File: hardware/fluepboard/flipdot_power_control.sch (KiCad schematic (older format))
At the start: 6 parts, among them IC3 SI4835DDY-T1-E3, Q2 BC847

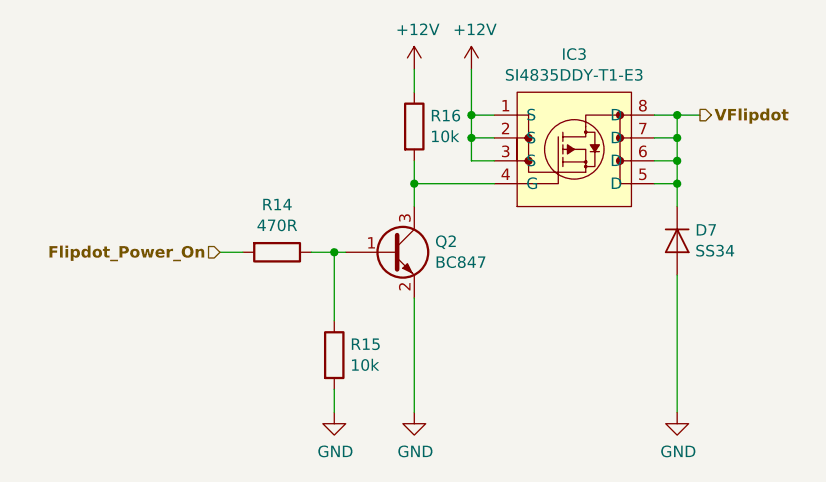
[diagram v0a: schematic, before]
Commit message: Commit jlcpcb compatible version
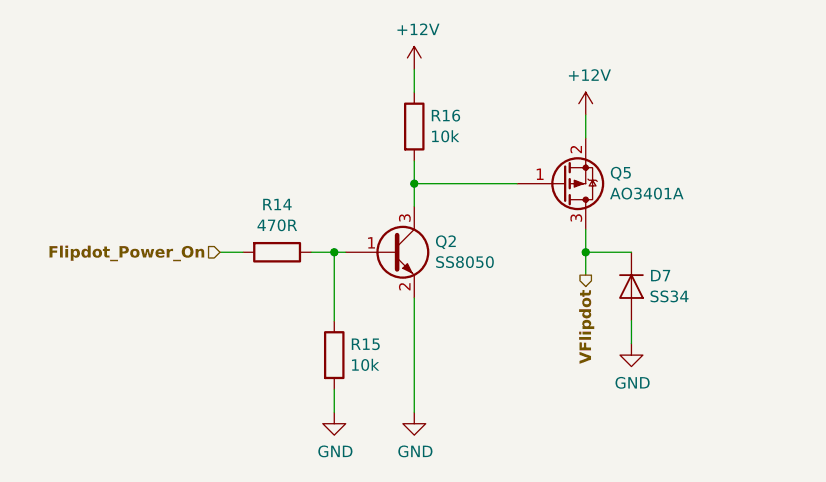
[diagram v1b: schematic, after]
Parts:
- removed IC3: SI4835DDY-T1-E3, Package_SO:SOIC-8_3.9x4.9mm_P1.27mm, symbol fluepdot:SI4835DDY-T1-E3
- removed Q2: BC847, Package_TO_SOT_SMD:SOT-23, symbol Transistor_BJT:BC847
- added Q2: SS8050, Package_TO_SOT_SMD:SOT-23, symbol Device:Q_NPN_BEC
- added Q5: AO3401A, Package_TO_SOT_SMD:SOT-23, symbol Device:Q_PMOS_GSD
- D7: footprint Diode_SMD:D_SMC -> Diode_SMD:D_SMA; Description (none) -> SCHOTTKY BARRIER DIODES (SBD) SMA(DO-214AC) ROHS; Extended Part (none) -> 0; LCSC (none) -> C84635; Manufacturer (none) -> SS34
- R14: footprint Resistor_SMD:R_0805_2012Metric -> Resistor_SMD:R_0603_1608Metric; Description (none) -> CHIP RESISTOR - SURFACE MOUNT 470OHMS ±1% 1/10W 0603 ROHS; Extended Part (none) -> 0; LCSC (none) -> C23179; Manufacturer (none) -> 0603WAF4700T5E
- R15, R16: footprint Resistor_SMD:R_0805_2012Metric -> Resistor_SMD:R_0603_1608Metric; Description (none) -> CHIP RESISTOR - SURFACE MOUNT 10KOHMS ±1% 1/10W 0603 ROHS; Extended Part (none) -> 0; LCSC (none) -> C25804; Manufacturer (none) -> 0603WAF1002T5E
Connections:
- net +12V: now also Q5.2 (S)
- net GND: now also Q2.2 (E)
- net VFlipdot: now also Q5.3 (D)
- net at R14.1, R15.1: now also Q2.1 (B)
- net at R16.2: now also Q2.3 (C), Q5.1 (G)
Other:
- moved on the sheet: D7
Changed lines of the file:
@@
 EESchema Schematic File Version 4
 LIBS:fluepdot-cache
-EELAYER 29 0
+EELAYER 30 0
 EELAYER END
 $Descr A4 11693 8268
@@
 $EndDescr
 $Comp
-L power:+12V #PWR?
-U 1 1 5CB72A62
-P 2500 850
-AR Path="/5CB72A62" Ref="#PWR?"  Part="1"
-AR Path="/5CA94BFB/5CB652B2/5CB72A62" Ref="#PWR?"  Part="1"
-F 0 "#PWR?" H 2500 700 50  0001 C CNN
-F 1 "+12V" H 2515 1023 50  0000 C CNN
-F 2 "" H 2500 850 50  0001 C CNN
-F 3 "" H 2500 850 50  0001 C CNN
-	1    2500 850
-	1    0    0    -1
-$EndComp
-Wire Wire Line
-	2500 850  2500 1050
-Wire Wire Line
-	2500 1250 2600 1250
-Wire Wire Line
-	2500 1150 2600 1150
-Connection ~ 2500 1150
-Wire Wire Line
-	2500 1150 2500 1250
-Wire Wire Line
-	2500 1050 2600 1050
-Connection ~ 2500 1050
-Wire Wire Line
-	2500 1050 2500 1150
-Wire Wire Line
-	3300 1050 3400 1050
-Wire Wire Line
-	3400 1050 3400 1150
-Wire Wire Line
-	3300 1150 3400 1150
-Connection ~ 3400 1150
-Wire Wire Line
-	3400 1150 3400 1250
-Wire Wire Line
-	3300 1250 3400 1250
-Connection ~ 3400 1250
-Wire Wire Line
-	3400 1250 3400 1350
-Wire Wire Line
-	3300 1350 3400 1350
-Connection ~ 3400 1350
-$Comp
-L Transistor_BJT:BC847 Q?
-U 1 1 5CB72A7B
-P 2150 1650
-AR Path="/5CB72A7B" Ref="Q?"  Part="1"
-AR Path="/5CA94BFB/5CB652B2/5CB72A7B" Ref="Q2"  Part="1"
-F 0 "Q2" H 2341 1696 50  0000 L CNN
-F 1 "BC847" H 2341 1605 50  0000 L CNN
-F 2 "Package_TO_SOT_SMD:SOT-23" H 2350 1575 50  0001 L CIN
-F 3 "http://www.infineon.com/dgdl/Infineon-BC847SERIES_BC848SERIES_BC849SERIES_BC850SERIES-DS-v01_01-en.pdf?fileId=db3a304314dca389011541d4630a1657" H 2150 1650 50  0001 L CNN
-F 4 "BC847,215" H 2150 1650 50  0001 C CNN "Octopart"
-	1    2150 1650
-	1    0    0    -1
-$EndComp
-$Comp
 L Device:R R?
 U 1 1 5CB72A81
@@
 F 0 "R16" H 2320 1146 50  0000 L CNN
 F 1 "10k" H 2320 1055 50  0000 L CNN
-F 2 "Resistor_SMD:R_0805_2012Metric" V 2180 1100 50  0001 C CNN
+F 2 "Resistor_SMD:R_0603_1608Metric" V 2180 1100 50  0001 C CNN
 F 3 "~" H 2250 1100 50  0001 C CNN
 F 4 "RC0805FR-0710KL" H 2250 1100 50  0001 C CNN "Octopart"
+F 5 "C25804" H 2250 1100 50  0001 C CNN "LCSC"
+F 6 "0603WAF1002T5E" H 2250 1100 50  0001 C CNN "Manufacturer"
+F 7 "0" H 2250 1100 50  0001 C CNN "Extended Part"
+F 8 "CHIP RESISTOR - SURFACE MOUNT 10KOHMS ±1% 1/10W 0603 ROHS" H 2250 1100 50  0001 C CNN "Description"
 	1    2250 1100
 	1    0    0    -1
@@
 Wire Wire Line
 	2250 1250 2250 1350
-Wire Wire Line
-	2250 1350 2600 1350
 Connection ~ 2250 1350
 Wire Wire Line
@@
 F 0 "R14" V 1443 1650 50  0000 C CNN
 F 1 "470R" V 1534 1650 50  0000 C CNN
-F 2 "Resistor_SMD:R_0805_2012Metric" V 1580 1650 50  0001 C CNN
+F 2 "Resistor_SMD:R_0603_1608Metric" V 1580 1650 50  0001 C CNN
 F 3 "~" H 1650 1650 50  0001 C CNN
 F 4 "RC0805FR-07470RL" H 1650 1650 50  0001 C CNN "Octopart"
+F 5 "0" H 1650 1650 50  0001 C CNN "Extended Part"
+F 6 "C23179" H 1650 1650 50  0001 C CNN "LCSC"
+F 7 "0603WAF4700T5E" H 1650 1650 50  0001 C CNN "Manufacturer"
+F 8 "CHIP RESISTOR - SURFACE MOUNT 470OHMS ±1% 1/10W 0603 ROHS" H 1650 1650 50  0001 C CNN "Description"
 	1    1650 1650
 	0    1    1    0
@@
 L Device:D D7
 U 1 1 5CB7BDC5
-P 3400 1600
-F 0 "D7" V 3354 1679 50  0000 L CNN
-F 1 "SS34" V 3445 1679 50  0000 L CNN
-F 2 "Diode_SMD:D_SMC" H 3400 1600 50  0001 C CNN
-F 3 "~" H 3400 1600 50  0001 C CNN
-F 4 "SS34-E3/57T" H 3400 1600 50  0001 C CNN "Octopart"
-	1    3400 1600
+P 3200 1800
+F 0 "D7" V 3154 1879 50  0000 L CNN
+F 1 "SS34" V 3245 1879 50  0000 L CNN
+F 2 "Diode_SMD:D_SMA" H 3200 1800 50  0001 C CNN
+F 3 "~" H 3200 1800 50  0001 C CNN
+F 4 "SS34-E3/57T" H 3200 1800 50  0001 C CNN "Octopart"
+F 5 "0" H 3200 1800 50  0001 C CNN "Extended Part"
+F 6 "C84635" H 3200 1800 50  0001 C CNN "LCSC"
+F 7 "SS34" H 3200 1800 50  0001 C CNN "Manufacturer"
+F 8 "SCHOTTKY BARRIER DIODES (SBD) SMA(DO-214AC) ROHS" H 3200 1800 50  0001 C CNN "Description"
+	1    3200 1800
 	0    1    1    0
 $EndComp
-Wire Wire Line
-	3400 1450 3400 1350
 $Comp
 L power:GND #PWR?
 U 1 1 5CB7C83D
-P 3400 2350
-F 0 "#PWR?" H 3400 2100 50  0001 C CNN
-F 1 "GND" H 3405 2177 50  0000 C CNN
-F 2 "" H 3400 2350 50  0001 C CNN
-F 3 "" H 3400 2350 50  0001 C CNN
-	1    3400 2350
-	1    0    0    -1
-$EndComp
-Wire Wire Line
-	3400 2350 3400 1750
+P 3200 2050
+F 0 "#PWR?" H 3200 1800 50  0001 C CNN
+F 1 "GND" H 3205 1877 50  0000 C CNN
+F 2 "" H 3200 2050 50  0001 C CNN
+F 3 "" H 3200 2050 50  0001 C CNN
+	1    3200 2050
+	1    0    0    -1
+$EndComp
 Wire Wire Line
 	1400 1650 1500 1650
-Text HLabel 3500 1050 2    50   Output ~ 10
+Text HLabel 3000 1750 3    50   Output ~ 10
 VFlipdot
-Wire Wire Line
-	3400 1050 3500 1050
-Connection ~ 3400 1050
 Text HLabel 1400 1650 0    50   Input ~ 10
 Flipdot_Power_On
@@
 F 0 "R15" H 1970 2146 50  0000 L CNN
 F 1 "10k" H 1970 2055 50  0000 L CNN
-F 2 "Resistor_SMD:R_0805_2012Metric" V 1830 2100 50  0001 C CNN
+F 2 "Resistor_SMD:R_0603_1608Metric" V 1830 2100 50  0001 C CNN
 F 3 "~" H 1900 2100 50  0001 C CNN
 F 4 "RC0805FR-0710KL" H 1900 2100 50  0001 C CNN "Octopart"
+F 5 "C25804" H 1900 2100 50  0001 C CNN "LCSC"
+F 6 "0603WAF1002T5E" H 1900 2100 50  0001 C CNN "Manufacturer"
+F 7 "0" H 1900 2100 50  0001 C CNN "Extended Part"
+F 8 "CHIP RESISTOR - SURFACE MOUNT 10KOHMS ±1% 1/10W 0603 ROHS" H 1900 2100 50  0001 C CNN "Description"
 	1    1900 2100
-	1    0    0    -1
-$EndComp
-$Comp
-L fluepdot:SI4835DDY-T1-E3 IC3
-U 1 1 5CC04B9C
-P 2950 1200
-F 0 "IC3" H 2950 1615 50  0000 C CNN
-F 1 "SI4835DDY-T1-E3" H 2950 1524 50  0000 C CNN
-F 2 "Package_SO:SOIC-8_3.9x4.9mm_P1.27mm" H 2950 1200 50  0001 C CNN
-F 3 "" H 2950 1200 50  0001 C CNN
-F 4 "SI4835DDY-T1-E3" H 2950 1200 50  0001 C CNN "Octopart"
-	1    2950 1200
 	1    0    0    -1
 $EndComp
@@
 Wire Wire Line
 	2250 1850 2250 2350
+Wire Wire Line
+	3000 1550 3000 1650
+Wire Wire Line
+	3200 1650 3000 1650
+Connection ~ 3000 1650
+Wire Wire Line
+	3000 1650 3000 1750
+Wire Wire Line
+	3200 1950 3200 2050
+$Comp
+L power:+12V #PWR?
+U 1 1 5D90ADB6
+P 3000 1050
+AR Path="/5D90ADB6" Ref="#PWR?"  Part="1"
+AR Path="/5CA94BFB/5CB652B2/5D90ADB6" Ref="#PWR?"  Part="1"
+F 0 "#PWR?" H 3000 900 50  0001 C CNN
+F 1 "+12V" H 3015 1223 50  0000 C CNN
+F 2 "" H 3000 1050 50  0001 C CNN
+F 3 "" H 3000 1050 50  0001 C CNN
+	1    3000 1050
+	1    0    0    -1
+$EndComp
+Wire Wire Line
+	3000 1050 3000 1150
+$Comp
+L Device:Q_PMOS_GSD Q5
+U 1 1 5D90586C
+P 2900 1350
+F 0 "Q5" H 3106 1304 50  0000 L CNN
+F 1 "AO3401A" H 3106 1395 50  0000 L CNN
+F 2 "Package_TO_SOT_SMD:SOT-23" H 3100 1450 50  0001 C CNN
+F 3 "~" H 2900 1350 50  0001 C CNN
+F 4 "0" H 2900 1350 50  0001 C CNN "Extended Part"
+F 5 "C15127" H 2900 1350 50  0001 C CNN "LCSC"
+F 6 "AO3401A" H 2900 1350 50  0001 C CNN "Manufacturer"
+F 7 "MOSFET P TRENCH 30V 4A 1.3V @ 250UA 44 M? @ 4.3A,10V SOT-23-3L ROHS" H 2900 1350 50  0001 C CNN "Description"
+	1    2900 1350
+	1    0    0    1
+$EndComp
+Wire Wire Line
+	2250 1350 2700 1350
+$Comp
+L Device:Q_NPN_BEC Q2
+U 1 1 5D9AFD81
+P 2150 1650
+F 0 "Q2" H 2341 1696 50  0000 L CNN
+F 1 "SS8050" H 2341 1605 50  0000 L CNN
+F 2 "Package_TO_SOT_SMD:SOT-23" H 2350 1750 50  0001 C CNN
+F 3 "~" H 2150 1650 50  0001 C CNN
+F 4 "TRANSISTORS (NPN/PNP) NPN 1.5A 25V SOT-23(SOT-23-3) ROHS" H 2150 1650 50  0001 C CNN "Description"
+F 5 "0" H 2150 1650 50  0001 C CNN "Extended Part"
+F 6 "C2150" H 2150 1650 50  0001 C CNN "LCSC"
+	1    2150 1650
+	1    0    0    -1
+$EndComp
 $EndSCHEMATC
